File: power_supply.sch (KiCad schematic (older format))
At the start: 33 parts, among them J1 Conn_01x01, J2 Conn_01x01, P0 10K, P1 100, Q1 BUT11A, Q2 BC547, SW1 SW_Rotary2x6, T1 Transformer_1P_6S, U1 L200, U2 LM317_3PinPackage

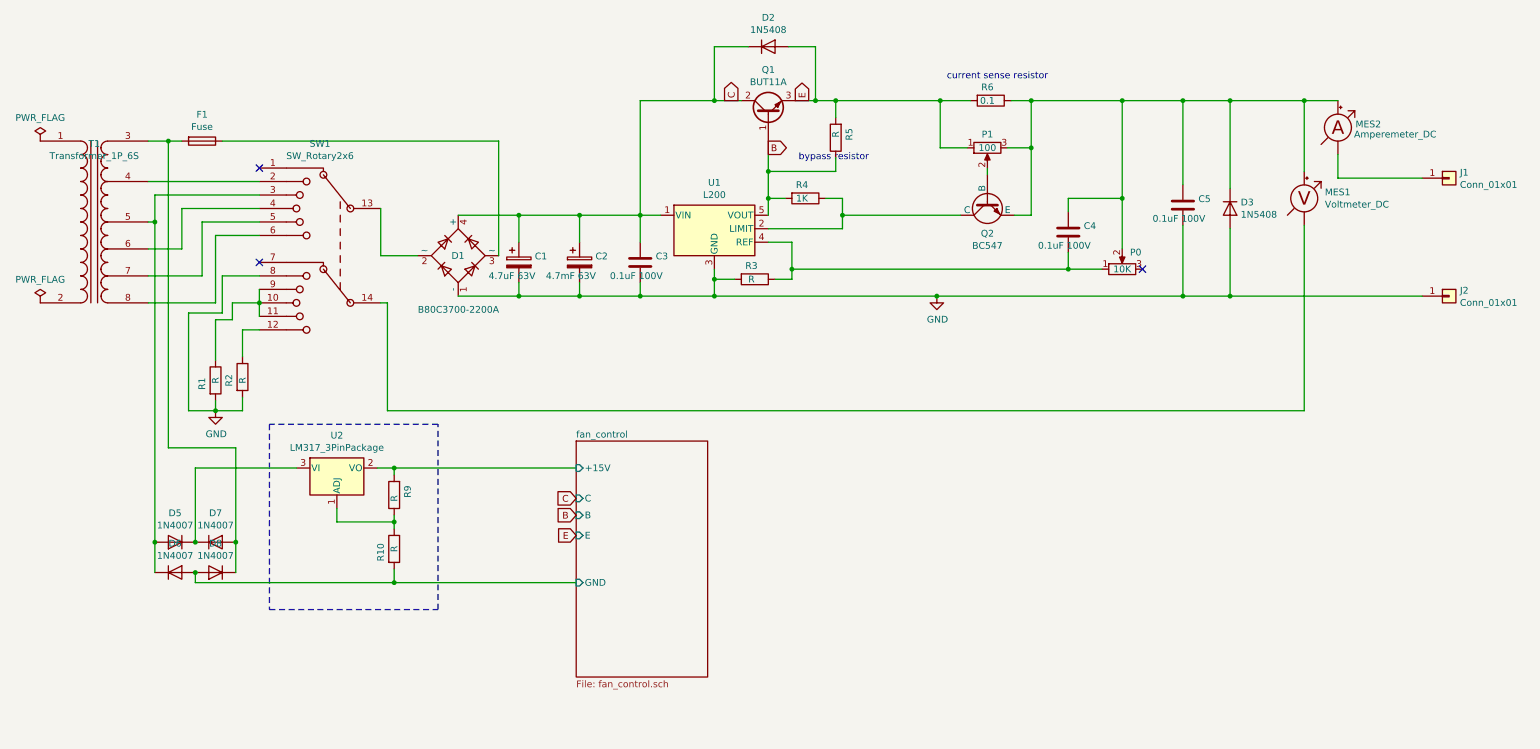
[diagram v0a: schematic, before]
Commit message: footprint assoziation; pcb layout; and more
* delete mainboard pcb
* rearrange project files/names
* create pcb layout
* improve schematics
* more
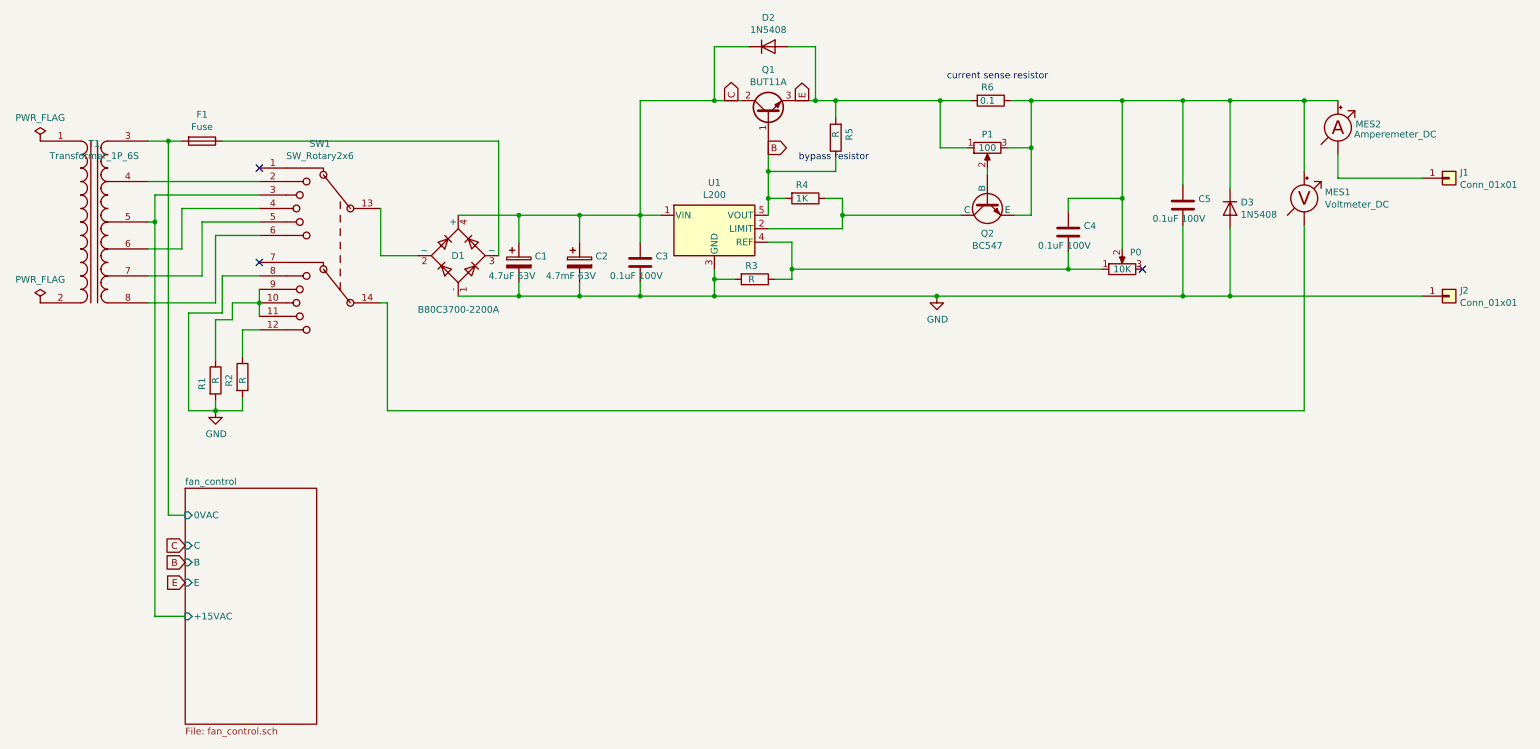
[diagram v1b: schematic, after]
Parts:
- removed D5, D6, D7, D8: 1N4007, Diode_THT:D_DO-41_SOD81_P2.54mm_Vertical_AnodeUp, symbol Diode:1N4007
- removed R10, R9: R, Resistor_THT:R_Axial_DIN0207_L6.3mm_D2.5mm_P2.54mm_Vertical, symbol Device:R
- removed U2: LM317_3PinPackage, Package_TO_SOT_THT:TO-220-3_Vertical, symbol Regulator_Linear:LM317_3PinPackage
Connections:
- net fan_control/0VAC: now reaches F1.2, T1.3 (SB)
- net fan_control/+15VAC: now reaches SW1.3, T1.5 (SC)
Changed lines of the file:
@@
 $EndComp
 $Sheet
-S 4525 4150 975  1750
+S 1625 4500 975  1750
 U 5E5C406E
 F0 "fan_control" 50
 F1 "fan_control.sch" 50
-F2 "GND" I L 4525 5200 50
-F3 "C" I L 4525 4575 50
-F4 "B" I L 4525 4700 50
-F5 "E" I L 4525 4850 50
-F6 "+15V" I L 4525 4350 50
+F2 "C" I L 1625 4925 50
+F3 "B" I L 1625 5050 50
+F4 "E" I L 1625 5200 50
+F5 "+15VAC" I L 1625 5450 50
+F6 "0VAC" I L 1625 4700 50
 $EndSheet
 NoConn ~ 2175 2125
@@
 $EndComp
 Wire Wire Line
-	1400 2525 1400 4900
+	1400 2525 1400 5450
 Connection ~ 1400 2525
-Wire Wire Line
-	1500 1925 1500 4200
 Connection ~ 1500 1925
 Wire Wire Line
 	1500 1925 1600 1925
-Wire Wire Line
-	1700 4350 2450 4350
-Wire Wire Line
-	2000 4200 1500 4200
-Wire Wire Line
-	1700 4350 1700 4900
-$Comp
-L Regulator_Linear:LM317_3PinPackage U2
-U 1 1 5E51FF6A
-P 2750 4350
-F 0 "U2" H 2750 4592 50  0000 C CNN
-F 1 "LM317_3PinPackage" H 2750 4501 50  0000 C CNN
-F 2 "Package_TO_SOT_THT:TO-220-3_Vertical" H 2750 4600 50  0001 C CIN
-F 3 "http://www.ti.com/lit/ds/symlink/lm317.pdf" H 2750 4350 50  0001 C CNN
-F 4 "N" H 2750 4350 50  0001 C CNN "Spice_Netlist_Enabled"
-	1    2750 4350
-	1    0    0    -1
-$EndComp
-$Comp
-L Device:R R10
-U 1 1 5E52057B
-P 3175 4950
-F 0 "R10" V 3075 4925 50  0000 C CNN
-F 1 "R" V 3175 4950 50  0000 C CNN
-F 2 "Resistor_THT:R_Axial_DIN0207_L6.3mm_D2.5mm_P2.54mm_Vertical" V 3105 4950 50  0001 C CNN
-F 3 "~" H 3175 4950 50  0001 C CNN
-F 4 "N" H 3175 4950 50  0001 C CNN "Spice_Netlist_Enabled"
-	1    3175 4950
-	1    0    0    -1
-$EndComp
-Wire Wire Line
-	3050 4350 3175 4350
-Wire Wire Line
-	3175 4750 2750 4750
-Wire Wire Line
-	2750 4750 2750 4650
-Wire Wire Line
-	3175 5100 3175 5200
-Connection ~ 3175 4750
-Wire Wire Line
-	3175 4750 3175 4800
-Wire Wire Line
-	3175 4350 3175 4400
-Wire Wire Line
-	3175 4750 3175 4700
-$Comp
-L Device:R R9
-U 1 1 5E5209D8
-P 3175 4550
-F 0 "R9" V 3075 4525 50  0000 C CNN
-F 1 "R" V 3175 4575 50  0000 C CNN
-F 2 "Resistor_THT:R_Axial_DIN0207_L6.3mm_D2.5mm_P2.54mm_Vertical" V 3105 4550 50  0001 C CNN
-F 3 "~" H 3175 4550 50  0001 C CNN
-F 4 "N" H 3175 4550 50  0001 C CNN "Spice_Netlist_Enabled"
-	1    3175 4550
-	-1   0    0    1
-$EndComp
-Connection ~ 3175 4350
 Text GLabel 6200 1625 1    50   Output ~ 0
 E
@@
 Wire Wire Line
 	4100 3075 4550 3075
-Text GLabel 4525 4575 0    50   Input ~ 0
+Text GLabel 1625 4925 0    50   Input ~ 0
 C
-Text GLabel 4525 4700 0    50   Input ~ 0
+Text GLabel 1625 5050 0    50   Input ~ 0
 B
-Text GLabel 4525 4850 0    50   Input ~ 0
+Text GLabel 1625 5200 0    50   Input ~ 0
 E
-Wire Wire Line
-	3175 5200 4525 5200
-Wire Wire Line
-	3175 4350 4525 4350
 Wire Wire Line
 	9375 3075 10800 3075
@@
 	1    0    0    -1
 $EndComp
-$Comp
-L Diode:1N4007 D5
-U 1 1 5E62A529
-P 1550 4900
-F 0 "D5" H 1550 4684 50  0000 C CNN
-F 1 "1N4007" H 1550 4775 50  0000 C CNN
-F 2 "Diode_THT:D_DO-41_SOD81_P2.54mm_Vertical_AnodeUp" H 1550 4725 50  0001 C CNN
-F 3 "http://www.vishay.com/docs/88503/1n4001.pdf" H 1550 4900 50  0001 C CNN
-F 4 "N" H 1550 4900 50  0001 C CNN "Spice_Netlist_Enabled"
-	1    1550 4900
-	-1   0    0    1
-$EndComp
-$Comp
-L Diode:1N4007 D7
-U 1 1 5E62B250
-P 1850 4900
-F 0 "D7" H 1850 5116 50  0000 C CNN
-F 1 "1N4007" H 1850 5025 50  0000 C CNN
-F 2 "Diode_THT:D_DO-41_SOD81_P2.54mm_Vertical_AnodeUp" H 1850 4725 50  0001 C CNN
-F 3 "http://www.vishay.com/docs/88503/1n4001.pdf" H 1850 4900 50  0001 C CNN
-F 4 "D" H 1850 4900 50  0001 C CNN "Spice_Primitive"
-F 5 "1N4007" H 1850 4900 50  0001 C CNN "Spice_Model"
-F 6 "N" H 1850 4900 50  0001 C CNN "Spice_Netlist_Enabled"
-	1    1850 4900
-	1    0    0    -1
-$EndComp
-$Comp
-L Diode:1N4007 D6
-U 1 1 5E63430D
-P 1550 5125
-F 0 "D6" H 1550 5341 50  0000 C CNN
-F 1 "1N4007" H 1550 5250 50  0000 C CNN
-F 2 "Diode_THT:D_DO-41_SOD81_P2.54mm_Vertical_AnodeUp" H 1550 4950 50  0001 C CNN
-F 3 "http://www.vishay.com/docs/88503/1n4001.pdf" H 1550 5125 50  0001 C CNN
-F 4 "N" H 1550 5125 50  0001 C CNN "Spice_Netlist_Enabled"
-	1    1550 5125
-	1    0    0    -1
-$EndComp
-Connection ~ 1700 4900
-$Comp
-L Diode:1N4007 D8
-U 1 1 5E64FCD6
-P 1850 5125
-F 0 "D8" H 1850 4909 50  0000 C CNN
-F 1 "1N4007" H 1850 5000 50  0000 C CNN
-F 2 "Diode_THT:D_DO-41_SOD81_P2.54mm_Vertical_AnodeUp" H 1850 4950 50  0001 C CNN
-F 3 "http://www.vishay.com/docs/88503/1n4001.pdf" H 1850 5125 50  0001 C CNN
-F 4 "N" H 1850 5125 50  0001 C CNN "Spice_Netlist_Enabled"
-	1    1850 5125
-	-1   0    0    1
-$EndComp
 Wire Wire Line
-	2000 4200 2000 4900
-Connection ~ 2000 4900
+	1400 5450 1625 5450
 Wire Wire Line
-	2000 4900 2000 5125
+	1625 4700 1500 4700
 Wire Wire Line
-	1400 4900 1400 5125
-Connection ~ 1400 4900
-Wire Wire Line
-	1700 5125 1700 5200
-Wire Wire Line
-	1700 5200 3175 5200
-Connection ~ 3175 5200
-Connection ~ 1700 5125
-Wire Notes Line
-	2250 4025 2250 5400
-Wire Notes Line
-	2250 5400 3500 5400
-Wire Notes Line
-	3500 5400 3500 4025
-Wire Notes Line
-	3500 4025 2250 4025
+	1500 1925 1500 4700
 $EndSCHEMATC
